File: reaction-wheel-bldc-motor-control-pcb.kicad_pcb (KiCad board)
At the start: 2 copper layers, 52.6 x 38.7 mm, 48 parts, among them J1 Conn_01x04_Pin, J2 Conn_01x04_Pin, J3 Conn_01x03_Pin, J4 USB_C_Receptacle_USB2.0_16P, J5 Conn_01x04_Pin, J6 Conn_01x06_Pin, SW1 SW_SPST, U1 USBLC6-2SC6, U2 STM32G431CBUx, U4 DRV8311H, U5 SN65HVD231, U6 TPS562200, Y1 16MHz

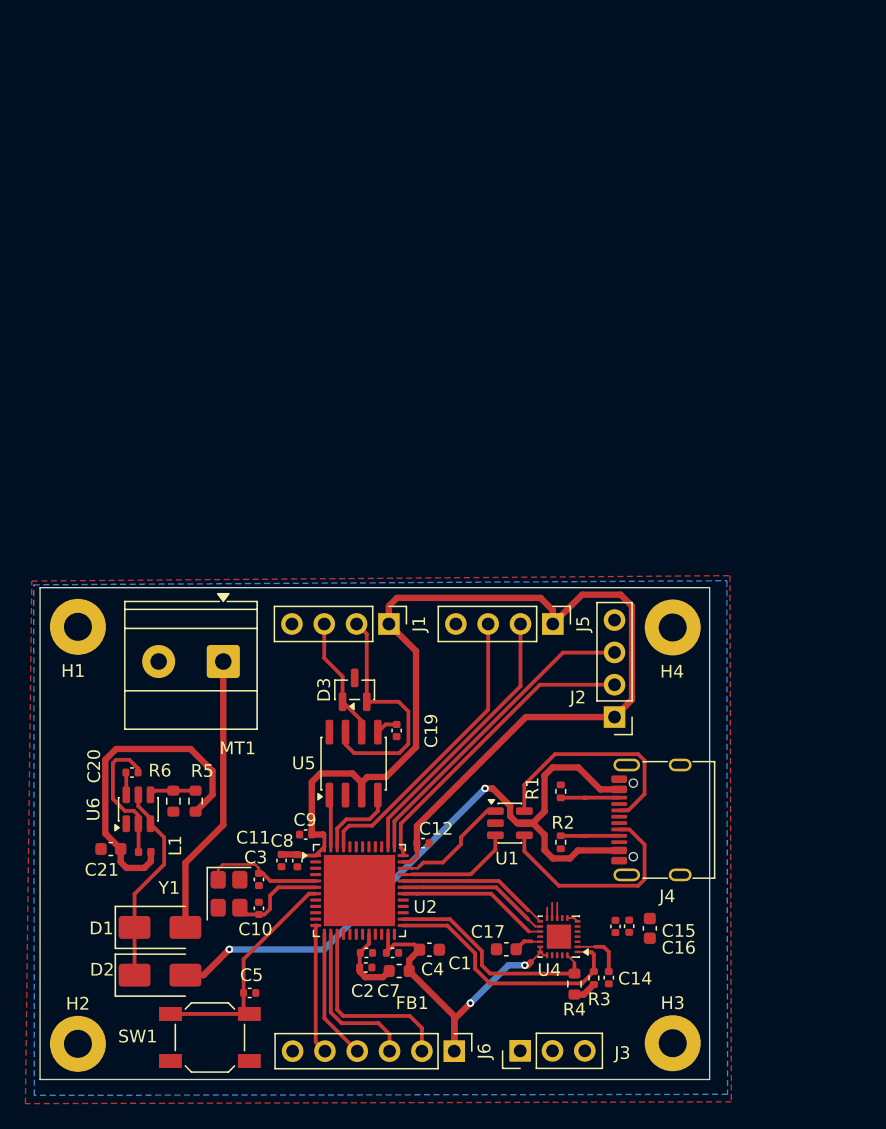
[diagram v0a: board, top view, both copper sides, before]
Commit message: routing almost finished
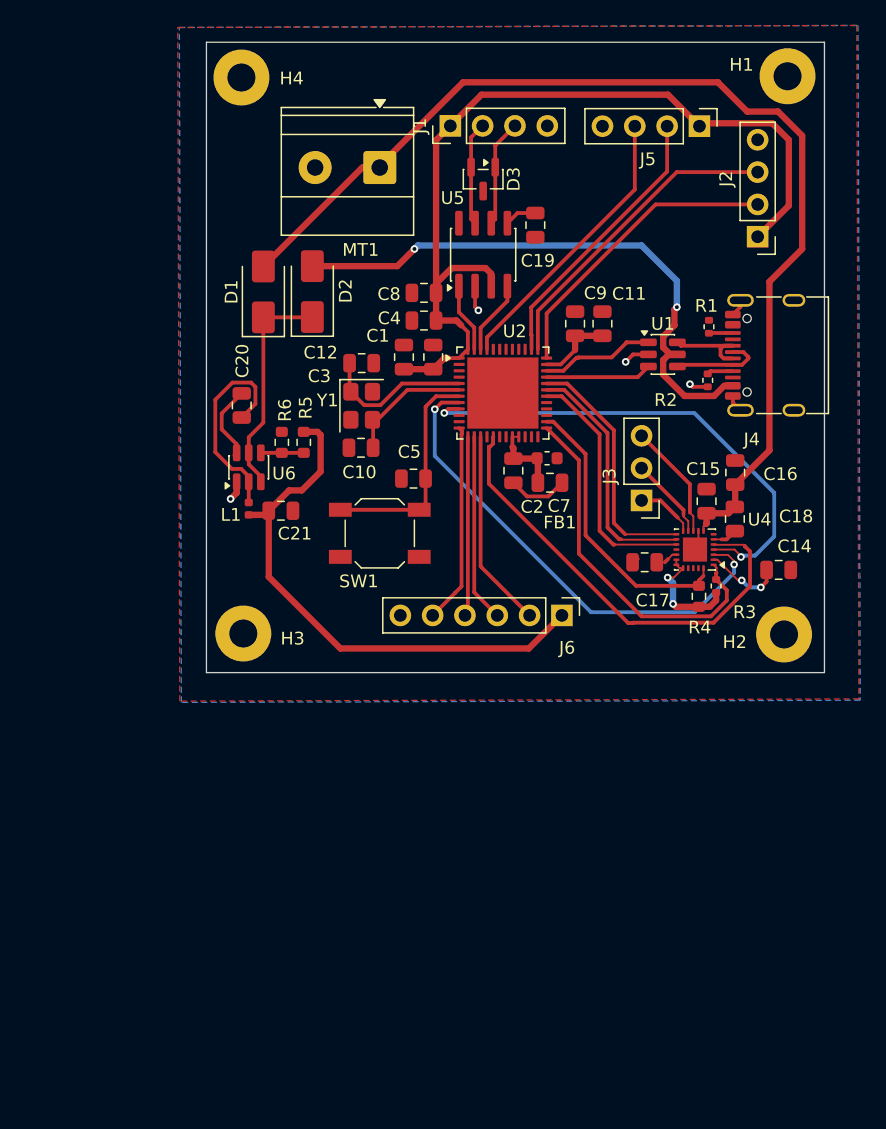
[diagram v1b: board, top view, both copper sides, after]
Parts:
- C1, C16, C17, C21: footprint Capacitor_SMD:C_0603_1608Metric -> Capacitor_SMD:C_0805_2012Metric
- C10, C11, C12, C14, C15, C18, C19, C2, C20, C3, C4, C5, C7, C8, C9: footprint Capacitor_SMD:C_0402_1005Metric -> Capacitor_SMD:C_0805_2012Metric
- moved H1 70.6 mm to (163.1, 67.1)
- moved H2 64.2 mm to (162.8, 111.0)
- moved D2 55.0 mm to (125.7, 84.0), turned to 90 degrees
- moved H4 54.9 mm to (120.1, 67.2)
- moved D1 50.6 mm to (121.8, 84.0), turned to 90 degrees
- moved C4 49.8 mm to (134.5, 86.3), turned to 180 degrees
- moved C11 49.2 mm to (148.5, 86.5), turned to 90 degrees
- moved H3 46.6 mm to (120.3, 110.9)
- moved C1 46.6 mm to (132.9, 89.2), turned to 90 degrees
- moved C8 45.7 mm to (134.5, 84.1), turned to 180 degrees
- moved C9 45.4 mm to (146.3, 86.5), turned to 90 degrees
- moved J3 44.3 mm to (151.6, 100.4), turned to 180 degrees
- moved C5 42.4 mm to (133.7, 98.7), turned to 0 degrees
- moved FB1 41.9 mm to (144.2, 97.1)
- moved SW1 41.8 mm to (131.0, 103.0)
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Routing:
- net VBAT: track 23.0 -> 85.5 mm
- net /PA1: track 0.00 -> 39.0 mm, vias 0 -> 2
- net /PA0: track 0.00 -> 38.4 mm, vias 0 -> 2
- net /PB0: track 0.00 -> 36.0 mm
- net GND: track 0.50 -> 16.7 mm, vias 0 -> 4
- net +3.3V: track 140.8 -> 128.7 mm
- net /CAN_H: track 19.1 -> 8.16 mm
- net /USBR_D+: track 18.0 -> 7.13 mm
- net /USBR_D-: track 17.3 -> 7.34 mm
- net +5V: track 54.8 -> 46.4 mm
- net /MOTOR_C: track 1.20 -> 9.16 mm
- net /FAULT: track 20.7 -> 28.4 mm
- net /PA8: track 12.0 -> 19.5 mm
- net /PA9: track 12.2 -> 19.5 mm
- net /PA10: track 12.1 -> 19.4 mm
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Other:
- board size 52.6 x 38.7 mm -> 48.6 x 49.5 mm
